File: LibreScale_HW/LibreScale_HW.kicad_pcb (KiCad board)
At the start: 2 copper layers, 52 x 68 mm, 22 parts, among them J1 AVR-UPDI-6, U1 ATtiny402-SS, U2 MCP3301, U3 INA333xxDGK

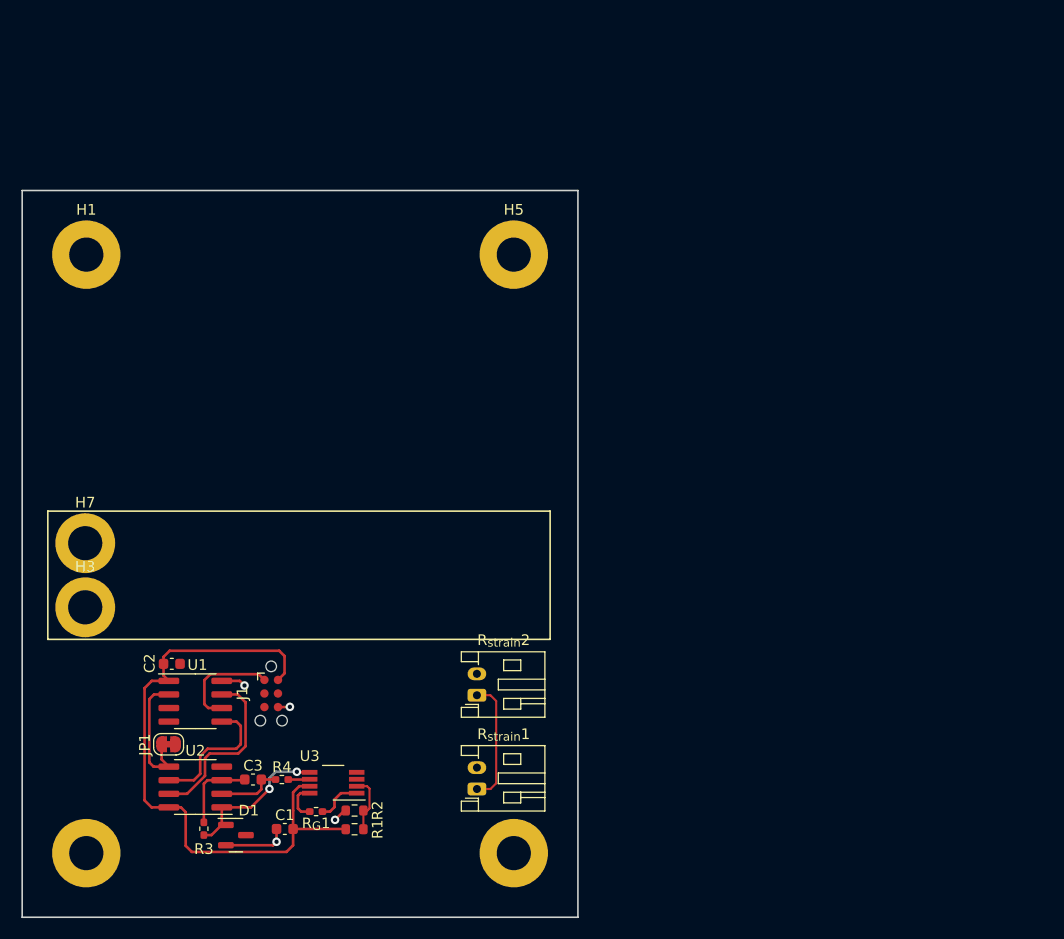
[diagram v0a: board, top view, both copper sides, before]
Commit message: Routing changes, added parts
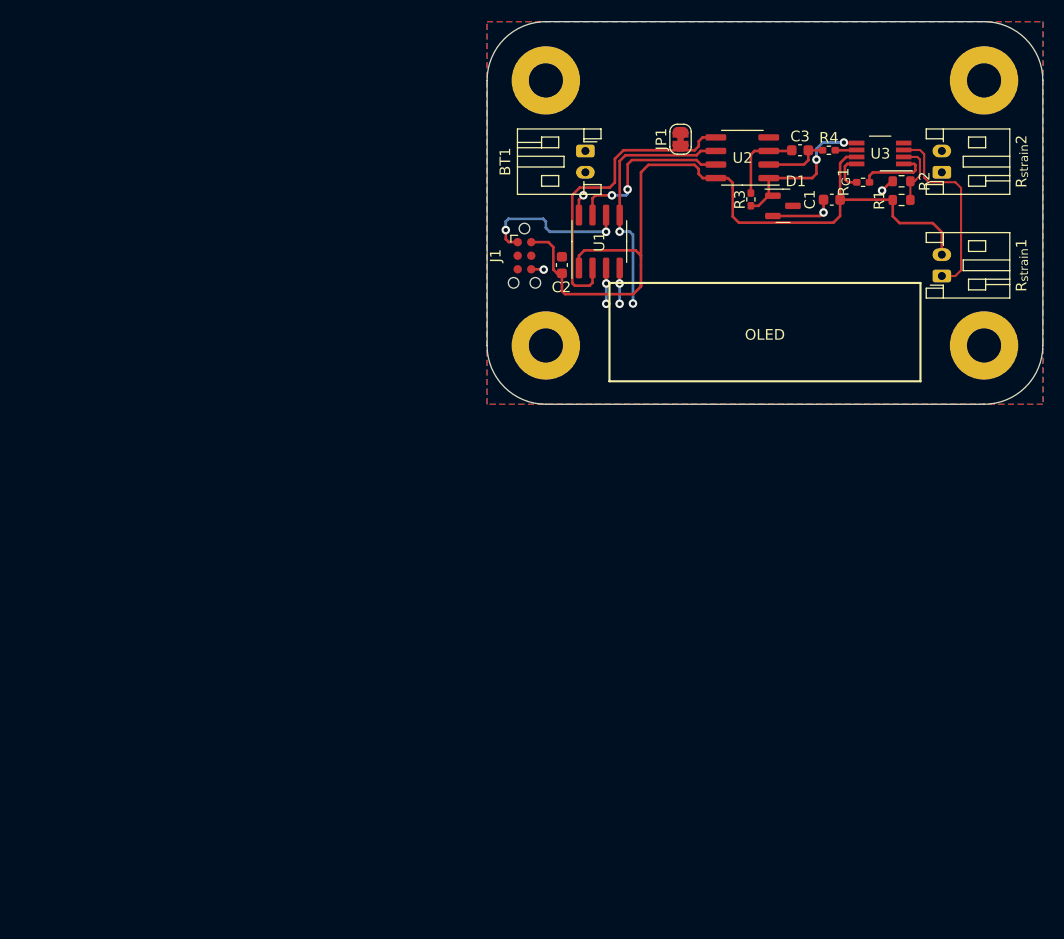
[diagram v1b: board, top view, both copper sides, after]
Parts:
- removed H3, H7: MountingHoleLoad, MountingHole:MountingHole_3.2mm_M3_DIN965_Pad
- added BT1: Battery_Cell, Connector_JST:JST_PH_S2B-PH-K_1x02_P2.00mm_Horizontal, F.Cu at (136.7, 100.3)
- moved R3 78.0 mm to (152.2, 104.8)
- moved C3 78.0 mm to (156.8, 100.2)
- moved D1 78.0 mm to (155.2, 105.4)
- moved R1 78.0 mm to (166.3, 104.9)
- moved R2 78.0 mm to (166.3, 103.1)
- moved R_{G}1 78.0 mm to (162.7, 103.2)
- moved U2 78.0 mm to (151.4, 100.9)
- moved U3 78.0 mm to (164.3, 100.5)
- moved C1 78.0 mm to (159.8, 104.9)
- moved R4 78.0 mm to (159.5, 100.2)
- moved JP1 74.2 mm to (145.6, 99.2), turned to -90 degrees
- moved R_{strain}2 65.5 mm to (170.1, 102.3)
- moved R_{strain}1 64.8 mm to (170.1, 112.0)
- moved H2 64.7 mm to (174.0, 118.5)
- moved H6 64.1 mm to (133.0, 118.5)
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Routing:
- net +5V: track 59.4 -> 77.2 mm
- net /CS1: track 12.3 -> 29.0 mm
- net /MISO: track 12.8 -> 23.8 mm, vias 0 -> 2
- net /V_{meas}+: track 11.7 -> 17.9 mm
- net /UDPI: track 10.1 -> 14.8 mm, vias 0 -> 2
- net /CS2: track 0.00 -> 3.38 mm, vias 0 -> 2
- net /MOSI: track 0.00 -> 3.38 mm, vias 0 -> 2
- net Net-(R_{G}1-Pad2): track 4.33 -> 6.75 mm
- net /V_{ref}: track 13.9 -> 14.7 mm
- net /SCK: track 16.6 -> 16.4 mm, vias 0 -> 2
- added copper zone on B.Cu, net GND
- added copper zone on F.Cu, net GND
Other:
- board size 52 x 68 mm -> 52 x 35.8 mm
- board text added: "LibreScale V0.1"
- board text added: "OLED"
